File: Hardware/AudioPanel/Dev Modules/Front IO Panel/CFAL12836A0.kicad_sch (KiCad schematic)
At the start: 3 parts, among them U301 CFAL12836A0-088

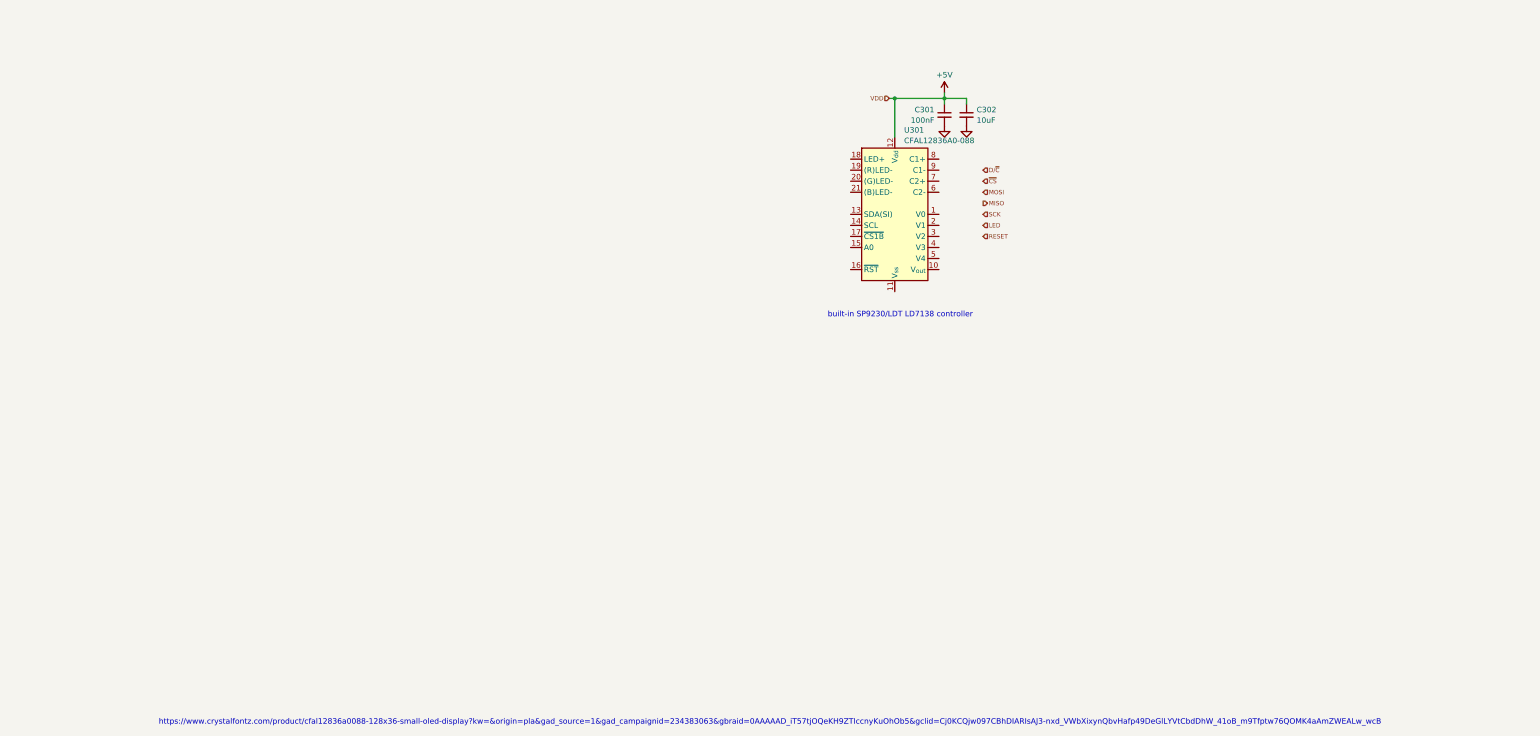
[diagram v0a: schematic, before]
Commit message: Work on front control panel
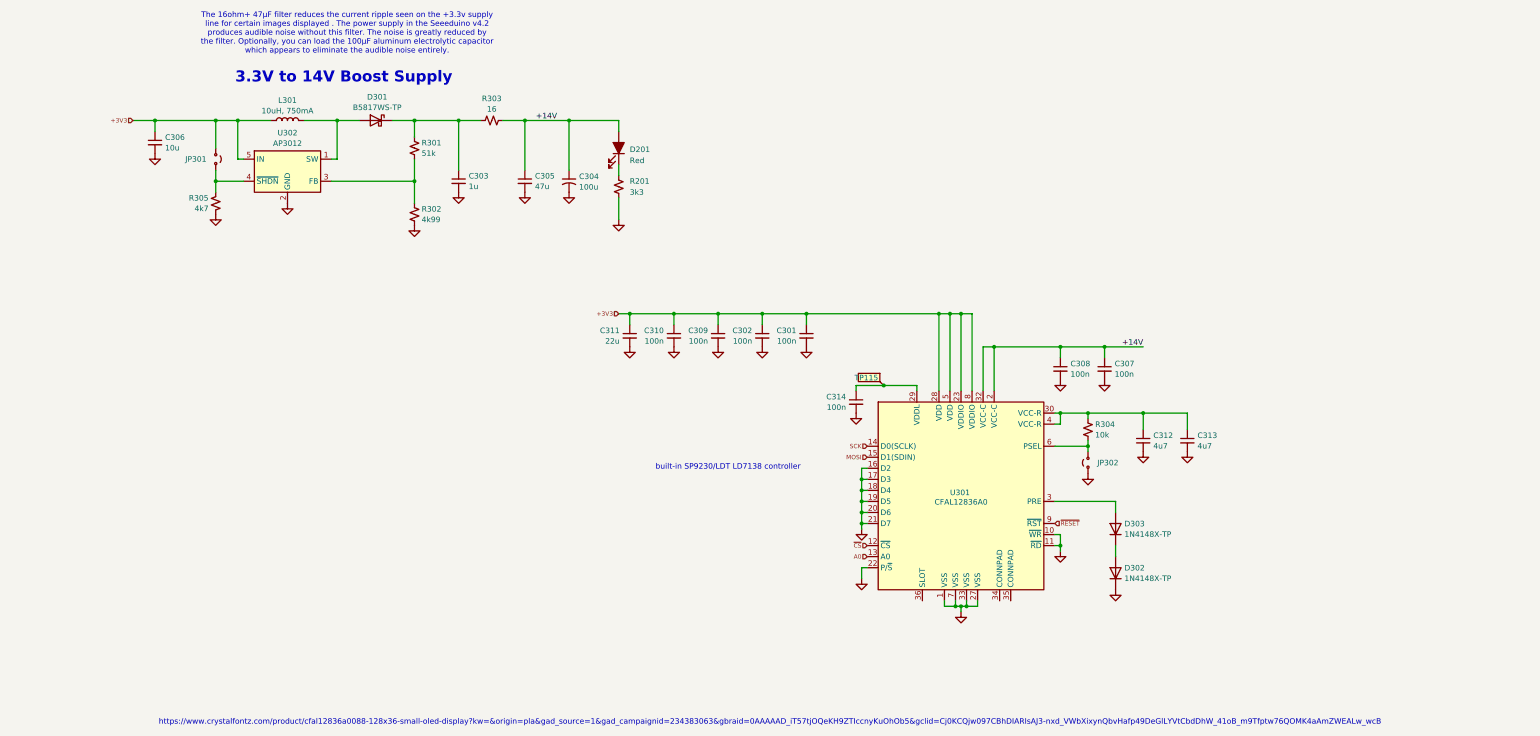
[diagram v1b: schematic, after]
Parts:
- removed U301: CFAL12836A0-088, Display:NHD-C12832A1Z-FSRGB, symbol Display_Graphic:NHD-C12832A1Z-FSRGB
- added C303: 1u, symbol Device:C_Small
- added C304: 100u, symbol Device:C_Small_US
- added C305: 47u, symbol Device:C_Small
- added C306: 10u, symbol Device:C_Small
- added C307, C308, C309, C310, C314: 100n, symbol Device:C_Small
- added C311: 22u, symbol Device:C_Small
- added C312, C313: 4u7, symbol Device:C_Small
- added D201: Red, LED_THT:LED_D5.0mm, symbol Device:LED_Filled
- added D301: B5817WS-TP, Diode_SMD:D_SOD-323, symbol Device:D_Schottky
- added D302, D303: 1N4148X-TP, Diode_SMD:D_SOD-523, symbol Device:D
- added JP301, JP302: Jumper_2_Small_Open, Jumper:SolderJumper-2_P1.3mm_Open_Pad1.0x1.5mm, symbol Jumper:Jumper_2_Small_Open
- added L301: 10uH, 750mA, symbol Device:L
- added R201: 3k3, Libraries:Worthington_R_0603, symbol Device:R_Small_US
- added R301: 51k, symbol Device:R_Small_US
- added R302: 4k99, symbol Device:R_Small_US
- added R303: 16, symbol Device:R_Small_US
- added R304: 10k, symbol Device:R_Small_US
- added R305: 4k7, symbol Device:R_Small_US
- added TP115: TestPoint_Flag, Libraries:KEYSTONE_5017, symbol Connector:TestPoint_Flag
- added U301: CFAL12836A0, Libraries:CFAL12836A0-088, symbol Libraries:CFAL12836A0
- added U302: AP3012, Package_TO_SOT_SMD:SOT-23-5, symbol Regulator_Switching:AP3012
- C301: value 100nF -> 100n
- C302: value 10uF -> 100n
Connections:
- net GND: now also C303.2, C304.2, C305.2, C306.2, C307.2, C308.2, C309.2, C310.2, C311.2, C312.2, C313.2, C314.2, D302.1 (K), JP302.1 (A), R201.1, R302.2, R305.2, U301.1 (VSS), U301.10 (~{WR}), U301.11 (~{RD}), U301.16 (D2), U301.17 (D3), U301.18 (D4), U301.19 (D5), U301.20 (D6), U301.21 (D7), U301.22 (P/~{S}), U301.27 (VSS), U301.33 (VSS), U301.7 (VSS), U302.2 (GND)
- net MOSI: now also U301.15 (D1(SDIN))
- net SCK: now also U301.14 (D0(SCLK))
- net ~{CS}: now also U301.12 (~{CS})
- net +5V renamed +3V3
- net +3V3: now also C306.1, C309.1, C310.1, C311.1, JP301.1 (A), L301.1, U301.23 (VDDIO), U301.28 (VDD), U301.5 (VDD), U301.8 (VDDIO), U302.5 (IN)
- new net: C303.1, D301.1 (K), R301.1, R303.1
- new net: D301.2 (A), L301.2, U302.1 (SW)
- new net: C314.1, TP115.1, U301.29 (VDDL)
- new net: C312.1, C313.1, R304.1, U301.30 (VCC-R), U301.4 (VCC-R)
- new net: JP302.2 (B), R304.2, U301.6 (PSEL)
- new net: JP301.2 (B), R305.1, U302.4 (~{SHDN})
- new net: R301.2, R302.1, U302.3 (FB)
- new net: D302.2 (A), D303.1 (K)
- new net: D201.1 (K), R201.2
- new net +14V: C304.1, C305.1, C307.1, C308.1, D201.2 (A), R303.2, U301.2 (VCC-C), U301.32 (VCC-C)
- new net A0: U301.13 (A0)
- new net PRE: D303.2 (A), U301.3 (PRE), U301.31 (PRE)
- new net ~{RESET}: U301.9 (~{RST})
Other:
- note added: "3.3V to 14V Boost Supply"
- note added: "The 16ohm+ 47µF filter reduces the current ripple seen on the +3.3v supply line for certain images displayed . The power supply in the Seeeduino v4.2 produces audible noise without this filter. The noise is greatly reduced by the filter. Optionally, you can load the 100µF aluminum electrolytic capacitor which appears to eliminate the audible noise entirely."
